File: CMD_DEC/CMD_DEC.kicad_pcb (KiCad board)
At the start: 2 copper layers, 76.2 x 54.6 mm, 24 parts, among them J1 Conn_01x04_Male, J10 Conn_01x01_Male, J11 Conn_01x01_Male, J12 Conn_01x01_Male, J13 Conn_01x01_Male, J14 Screw_Terminal_01x02, J2 Conn_01x01_Male, J3 Conn_01x05_Male, J4 Conn_01x08_Male, J5 Conn_01x08_Male, J6 Conn_01x02_Male, J7 Conn_01x01_Male, J8 Conn_01x01_Male, J9 Conn_01x01_Male, U1 74LS08, U2 74LS138, U3 74LS139, U4 74LS138, U5 74LS85, U6 74HC00

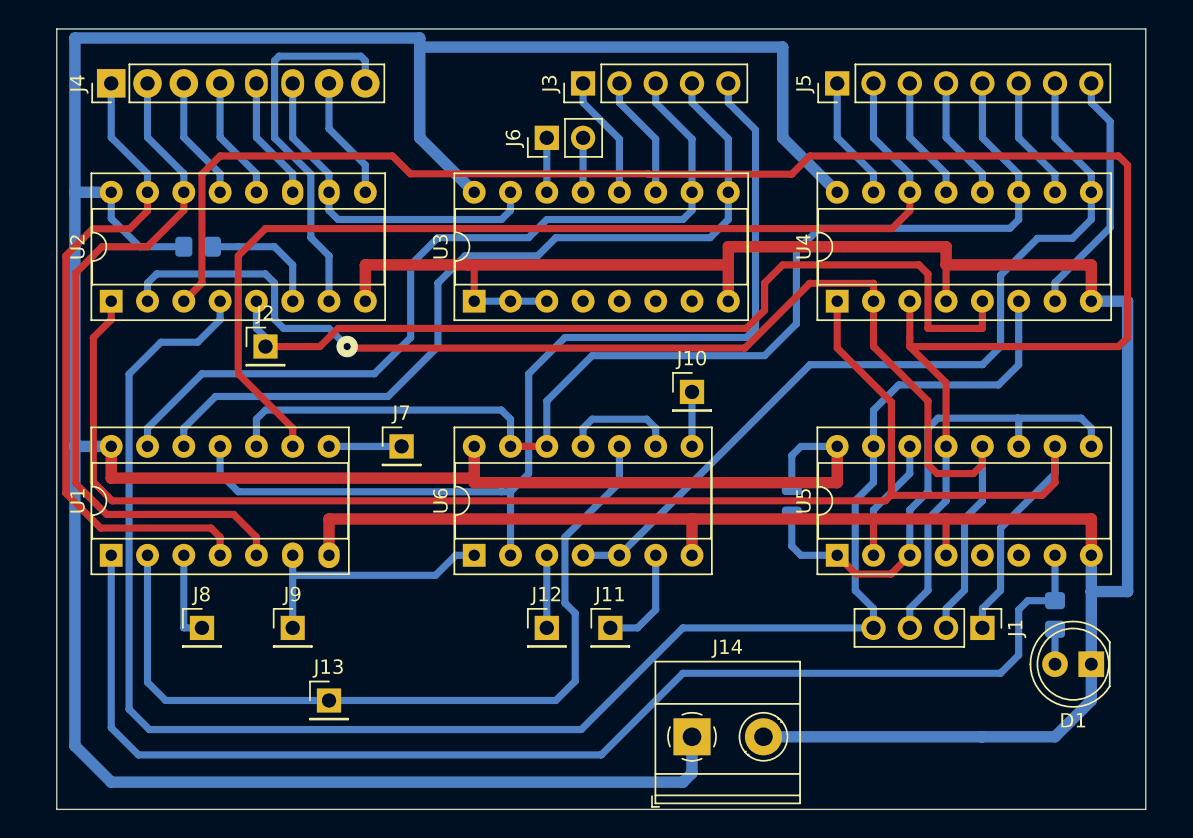
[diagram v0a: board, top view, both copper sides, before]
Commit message: Polishing Cmd dec
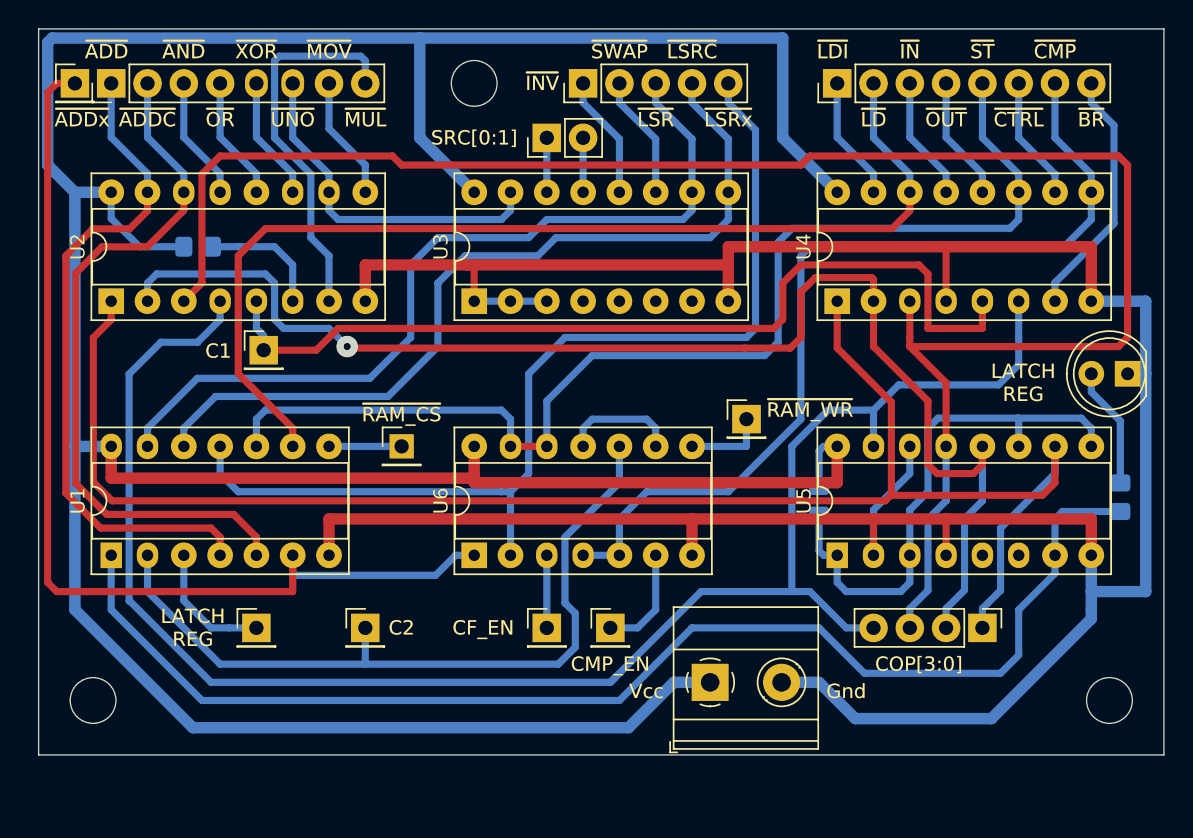
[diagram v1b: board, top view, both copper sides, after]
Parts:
- added H1: MountingHole, MountingHole:MountingHole_3.2mm_M3, F.Cu at (58.4, 33.0)
- added H2: MountingHole, MountingHole:MountingHole_3.2mm_M3, F.Cu at (102.9, 76.2)
- added H3: MountingHole, MountingHole:MountingHole_3.2mm_M3, F.Cu at (31.8, 76.2)
- moved J9 41.0 mm to (30.5, 33.0)
- moved D1 20.5 mm to (104.1, 53.3)
- moved R5 9.42 mm to (103.6, 62.0), turned to 90 degrees
- moved J13 5.68 mm to (50.8, 71.1)
- moved J10 4.26 mm to (77.5, 56.5)
- moved J14 4.02 mm to (74.9, 74.9)
- moved J8 3.81 mm to (43.2, 71.1)
- moved R2 1.91 mm to (82.5, 62.2)
- moved J2 0.28 mm to (43.7, 51.7)
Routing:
- net /~ADDx: track 18.4 -> 71.1 mm
- net Net-(D1-Pad2): track 2.44 -> 8.48 mm
- net VCC: track 246.7 -> 240.8 mm
- net /~CMP: track 58.8 -> 64.1 mm
- net /C2: track 58.2 -> 53.5 mm
- net /LATCH_REG: track 6.35 -> 9.04 mm
- net /COP[1]: track 91.5 -> 93.9 mm
- net /~RAM_WR: track 3.81 -> 5.72 mm
- net Net-(R2-Pad1): track 36.5 -> 38.0 mm
- net /COP[3]: track 120.5 -> 119.1 mm
- net /~ST: track 79.7 -> 80.8 mm
- net GND: track 205.5 -> 206.4 mm
- net /WILL_WR2REG: track 88.4 -> 89.3 mm
- net /C1: track 63.1 -> 63.9 mm
- net /COP[2]: track 128.6 -> 128.0 mm
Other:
- board size 76.2 x 54.6 mm -> 78.7 x 50.8 mm
- board text added: "C1"
- board text added: "C2"
- board text added: "CF_EN"
- board text added: "CMP_EN"
- board text added: "COP[3:0]"
- board text added: "Gnd"
- board text added: "LATCH REG"
- board text added: "SRC[0:1]"
- board text added: "Vcc"
- board text added: "~ADD"
- board text added: "~ADDC"
- board text added: "~ADDx"
- board text added: "~AND"
- board text added: "~BR"
- board text added: "~CMP"
- board text added: "~CTRL"
- board text added: "~IN"
- board text added: "~INV"
- board text added: "~LD"
- board text added: "~LDI"
- board text added: "~LSR"
- board text added: "~LSRC"
- board text added: "~LSRx"
- board text added: "~MOV"
- board text added: "~MUL"
- board text added: "~OR"
- board text added: "~OUT"
- board text added: "~RAM_CS"
- board text added: "~RAM_WR"
- board text added: "~ST"
- board text added: "~SWAP"
- board text added: "~UNO"
- board text added: "~XOR"
